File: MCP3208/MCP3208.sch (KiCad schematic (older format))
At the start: 33 parts, among them J1 5V, J2 SPI, J3 CH4, J4 CH3, J5 CH2, J6 CH1, U1 MCP1541, U2 MCP6021, U3 MCP3208

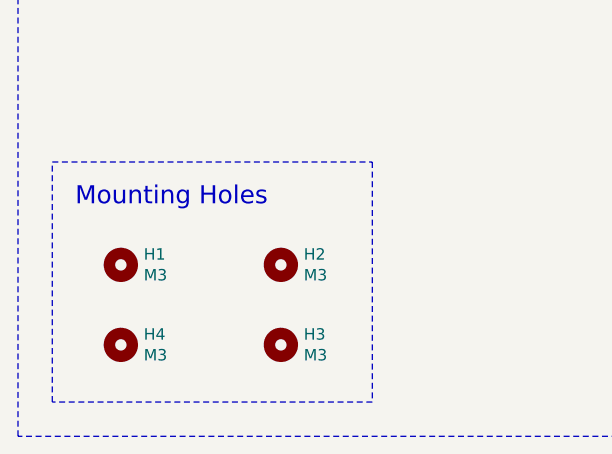
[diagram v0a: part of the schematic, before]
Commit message: Updates to schematic and PCB
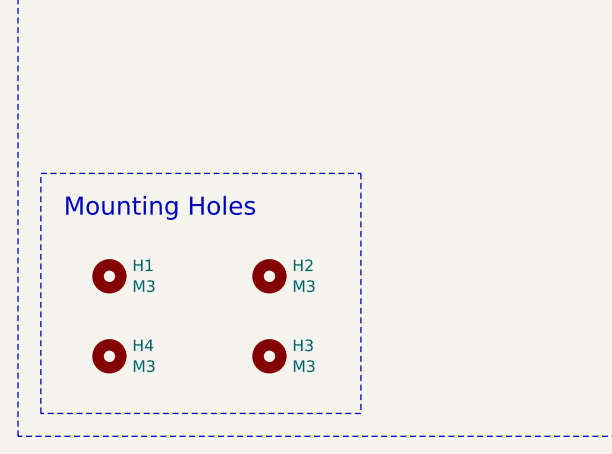
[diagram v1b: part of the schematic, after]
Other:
- moved on the sheet: H1, H2, H3, H4
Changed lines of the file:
@@
 L Mechanical:MountingHole H4
 U 1 1 60919793
-P 1600 6050
-F 0 "H4" H 1700 6096 50  0000 L CNN
-F 1 "M3" H 1700 6005 50  0000 L CNN
-F 2 "MountingHole:MountingHole_3.2mm_M3_ISO14580" H 1600 6050 50  0001 C CNN
-F 3 "~" H 1600 6050 50  0001 C CNN
-F 4 "~" H 1600 6050 50  0001 C CNN "Impedence "
-F 5 "~" H 1600 6050 50  0001 C CNN "MPN"
-F 6 "~" H 1600 6050 50  0001 C CNN "Manufacturer"
-F 7 "~" H 1600 6050 50  0001 C CNN "Power"
-F 8 "~" H 1600 6050 50  0001 C CNN "Rating"
-F 9 "~" H 1600 6050 50  0001 C CNN "Tolerance"
-	1    1600 6050
+P 1550 6100
+F 0 "H4" H 1650 6146 50  0000 L CNN
+F 1 "M3" H 1650 6055 50  0000 L CNN
+F 2 "MountingHole:MountingHole_3.2mm_M3_ISO14580" H 1550 6100 50  0001 C CNN
+F 3 "~" H 1550 6100 50  0001 C CNN
+F 4 "~" H 1550 6100 50  0001 C CNN "Impedence "
+F 5 "~" H 1550 6100 50  0001 C CNN "MPN"
+F 6 "~" H 1550 6100 50  0001 C CNN "Manufacturer"
+F 7 "~" H 1550 6100 50  0001 C CNN "Power"
+F 8 "~" H 1550 6100 50  0001 C CNN "Rating"
+F 9 "~" H 1550 6100 50  0001 C CNN "Tolerance"
+	1    1550 6100
 	1    0    0    -1
 $EndComp
@@
 L Mechanical:MountingHole H3
 U 1 1 6091947B
-P 2300 6050
-F 0 "H3" H 2400 6096 50  0000 L CNN
-F 1 "M3" H 2400 6005 50  0000 L CNN
-F 2 "MountingHole:MountingHole_3.2mm_M3_ISO14580" H 2300 6050 50  0001 C CNN
-F 3 "~" H 2300 6050 50  0001 C CNN
-F 4 "~" H 2300 6050 50  0001 C CNN "Impedence "
-F 5 "~" H 2300 6050 50  0001 C CNN "MPN"
-F 6 "~" H 2300 6050 50  0001 C CNN "Manufacturer"
-F 7 "~" H 2300 6050 50  0001 C CNN "Power"
-F 8 "~" H 2300 6050 50  0001 C CNN "Rating"
-F 9 "~" H 2300 6050 50  0001 C CNN "Tolerance"
-	1    2300 6050
+P 2250 6100
+F 0 "H3" H 2350 6146 50  0000 L CNN
+F 1 "M3" H 2350 6055 50  0000 L CNN
+F 2 "MountingHole:MountingHole_3.2mm_M3_ISO14580" H 2250 6100 50  0001 C CNN
+F 3 "~" H 2250 6100 50  0001 C CNN
+F 4 "~" H 2250 6100 50  0001 C CNN "Impedence "
+F 5 "~" H 2250 6100 50  0001 C CNN "MPN"
+F 6 "~" H 2250 6100 50  0001 C CNN "Manufacturer"
+F 7 "~" H 2250 6100 50  0001 C CNN "Power"
+F 8 "~" H 2250 6100 50  0001 C CNN "Rating"
+F 9 "~" H 2250 6100 50  0001 C CNN "Tolerance"
+	1    2250 6100
 	1    0    0    -1
 $EndComp
@@
 L Mechanical:MountingHole H2
 U 1 1 60919211
-P 2300 5700
-F 0 "H2" H 2400 5746 50  0000 L CNN
-F 1 "M3" H 2400 5655 50  0000 L CNN
-F 2 "MountingHole:MountingHole_3.2mm_M3_ISO14580" H 2300 5700 50  0001 C CNN
-F 3 "~" H 2300 5700 50  0001 C CNN
-F 4 "~" H 2300 5700 50  0001 C CNN "Impedence "
-F 5 "~" H 2300 5700 50  0001 C CNN "MPN"
-F 6 "~" H 2300 5700 50  0001 C CNN "Manufacturer"
-F 7 "~" H 2300 5700 50  0001 C CNN "Power"
-F 8 "~" H 2300 5700 50  0001 C CNN "Rating"
-F 9 "~" H 2300 5700 50  0001 C CNN "Tolerance"
-	1    2300 5700
+P 2250 5750
+F 0 "H2" H 2350 5796 50  0000 L CNN
+F 1 "M3" H 2350 5705 50  0000 L CNN
+F 2 "MountingHole:MountingHole_3.2mm_M3_ISO14580" H 2250 5750 50  0001 C CNN
+F 3 "~" H 2250 5750 50  0001 C CNN
+F 4 "~" H 2250 5750 50  0001 C CNN "Impedence "
+F 5 "~" H 2250 5750 50  0001 C CNN "MPN"
+F 6 "~" H 2250 5750 50  0001 C CNN "Manufacturer"
+F 7 "~" H 2250 5750 50  0001 C CNN "Power"
+F 8 "~" H 2250 5750 50  0001 C CNN "Rating"
+F 9 "~" H 2250 5750 50  0001 C CNN "Tolerance"
+	1    2250 5750
 	1    0    0    -1
 $EndComp
@@
 L Mechanical:MountingHole H1
 U 1 1 60918BE5
-P 1600 5700
-F 0 "H1" H 1700 5746 50  0000 L CNN
-F 1 "M3" H 1700 5655 50  0000 L CNN
-F 2 "MountingHole:MountingHole_3.2mm_M3_ISO14580" H 1600 5700 50  0001 C CNN
-F 3 "~" H 1600 5700 50  0001 C CNN
-F 4 "~" H 1600 5700 50  0001 C CNN "Impedence "
-F 5 "~" H 1600 5700 50  0001 C CNN "MPN"
-F 6 "~" H 1600 5700 50  0001 C CNN "Manufacturer"
-F 7 "~" H 1600 5700 50  0001 C CNN "Power"
-F 8 "~" H 1600 5700 50  0001 C CNN "Rating"
-F 9 "~" H 1600 5700 50  0001 C CNN "Tolerance"
-	1    1600 5700
+P 1550 5750
+F 0 "H1" H 1650 5796 50  0000 L CNN
+F 1 "M3" H 1650 5705 50  0000 L CNN
+F 2 "MountingHole:MountingHole_3.2mm_M3_ISO14580" H 1550 5750 50  0001 C CNN
+F 3 "~" H 1550 5750 50  0001 C CNN
+F 4 "~" H 1550 5750 50  0001 C CNN "Impedence "
+F 5 "~" H 1550 5750 50  0001 C CNN "MPN"
+F 6 "~" H 1550 5750 50  0001 C CNN "Manufacturer"
+F 7 "~" H 1550 5750 50  0001 C CNN "Power"
+F 8 "~" H 1550 5750 50  0001 C CNN "Rating"
+F 9 "~" H 1550 5750 50  0001 C CNN "Tolerance"
+	1    1550 5750
 	1    0    0    -1
 $EndComp
-Text Notes 1400 5450 0    79   ~ 0
+Text Notes 1350 5500 0    79   ~ 0
 Mounting Holes
 Wire Notes Line
-	1300 5250 2700 5250
+	1250 5300 2650 5300
 Wire Notes Line
-	2700 5250 2700 6300
+	2650 5300 2650 6350
 Wire Notes Line
-	2700 6300 1300 6300
+	2650 6350 1250 6350
 Wire Notes Line
-	1300 6300 1300 5250
+	1250 6350 1250 5300
 Connection ~ 3900 1500
 Wire Wire Line
